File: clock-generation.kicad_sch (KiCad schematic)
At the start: 0 parts

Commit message: wip
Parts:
- added U1: Si5351B-B-GM, Package_DFN_QFN:QFN-20-1EP_4x4mm_P0.5mm_EP2.7x2.7mm, symbol Oscillator:Si5351B-B-GM
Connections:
- new net SCL: U1.4 (SCL)
- new net SDA: U1.5 (SDA)
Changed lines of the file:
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@@
 	(generator_version "8.0")
 	(paper "A4")
+	(wire
+		(pts
+			(xy 92.71 83.82) (xy 121.92 83.82)
+		)
+		(stroke
+			(width 0)
+			(type default)
+		)
+	)
+	(wire
+		(pts
+			(xy 92.71 86.36) (xy 121.92 86.36)
+		)
+		(stroke
+			(width 0)
+			(type default)
+		)
+	)
+	(hierarchical_label "SCL"
+		(shape bidirectional)
+		(at 92.71 86.36 180)
+		(fields_autoplaced yes)
+		(effects
+			(font
+				(size 1.27 1.27)
+			)
+			(justify right)
+		)
+	)
+	(hierarchical_label "SDA"
+		(shape bidirectional)
+		(at 92.71 83.82 180)
+		(fields_autoplaced yes)
+		(effects
+			(font
+				(size 1.27 1.27)
+			)
+			(justify right)
+		)
+	)
+	(symbol
+		(lib_id "Oscillator:Si5351B-B-GM")
+		(at 137.16 78.74 0)
+		(unit 1)
+		(exclude_from_sim no)
+		(in_bom yes)
+		(on_board yes)
+		(dnp no)
+		(fields_autoplaced yes)
+		(property "Reference" "U1"
+			(at 139.3541 101.6 0)
+			(effects
+				(font
+					(size 1.27 1.27)
+				)
+				(justify left)
+			)
+		)
+		(property "Value" "Si5351B-B-GM"
+			(at 139.3541 104.14 0)
+			(effects
+				(font
+					(size 1.27 1.27)
+				)
+				(justify left)
+			)
+		)
+		(property "Footprint" "Package_DFN_QFN:QFN-20-1EP_4x4mm_P0.5mm_EP2.7x2.7mm"
+			(at 137.16 109.22 0)
+			(effects
+				(font
+					(size 1.27 1.27)
+				)
+				(hide yes)
+			)
+		)
+		(property "Datasheet" "https://www.silabs.com/documents/public/data-sheets/Si5351-B.pdf"
+			(at 137.16 78.74 0)
+			(effects
+				(font
+					(size 1.27 1.27)
+				)
+				(hide yes)
+			)
+		)
+		(property "Description" "I2C Programmable Any-Frequency CMOS Clock Generator + VCXO, QFN-20"
+			(at 137.16 78.74 0)
+			(effects
+				(font
+					(size 1.27 1.27)
+				)
+				(hide yes)
+			)
+		)
+		(pin "17"
+		)
+		(pin "21"
+		)
+		(pin "20"
+		)
+		(pin "2"
+		)
+		(pin "3"
+		)
+		(pin "9"
+		)
+		(pin "1"
+		)
+		(pin "13"
+		)
+		(pin "5"
+		)
+		(pin "7"
+		)
+		(pin "4"
+		)
+		(pin "6"
+		)
+		(pin "15"
+		)
+		(pin "10"
+		)
+		(pin "8"
+		)
+		(pin "14"
+		)
+		(pin "18"
+		)
+		(pin "11"
+		)
+		(pin "16"
+		)
+		(pin "12"
+		)
+		(pin "19"
+		)
+		(instances
+			(project ""
+				(path "/df100556-b288-4cb1-b69f-c0734132cb90/be7c4f40-c0c2-47f2-9c0c-8904af6555df"
+					(reference "U1")
+					(unit 1)
+				)
+			)
+		)
+	)
 )

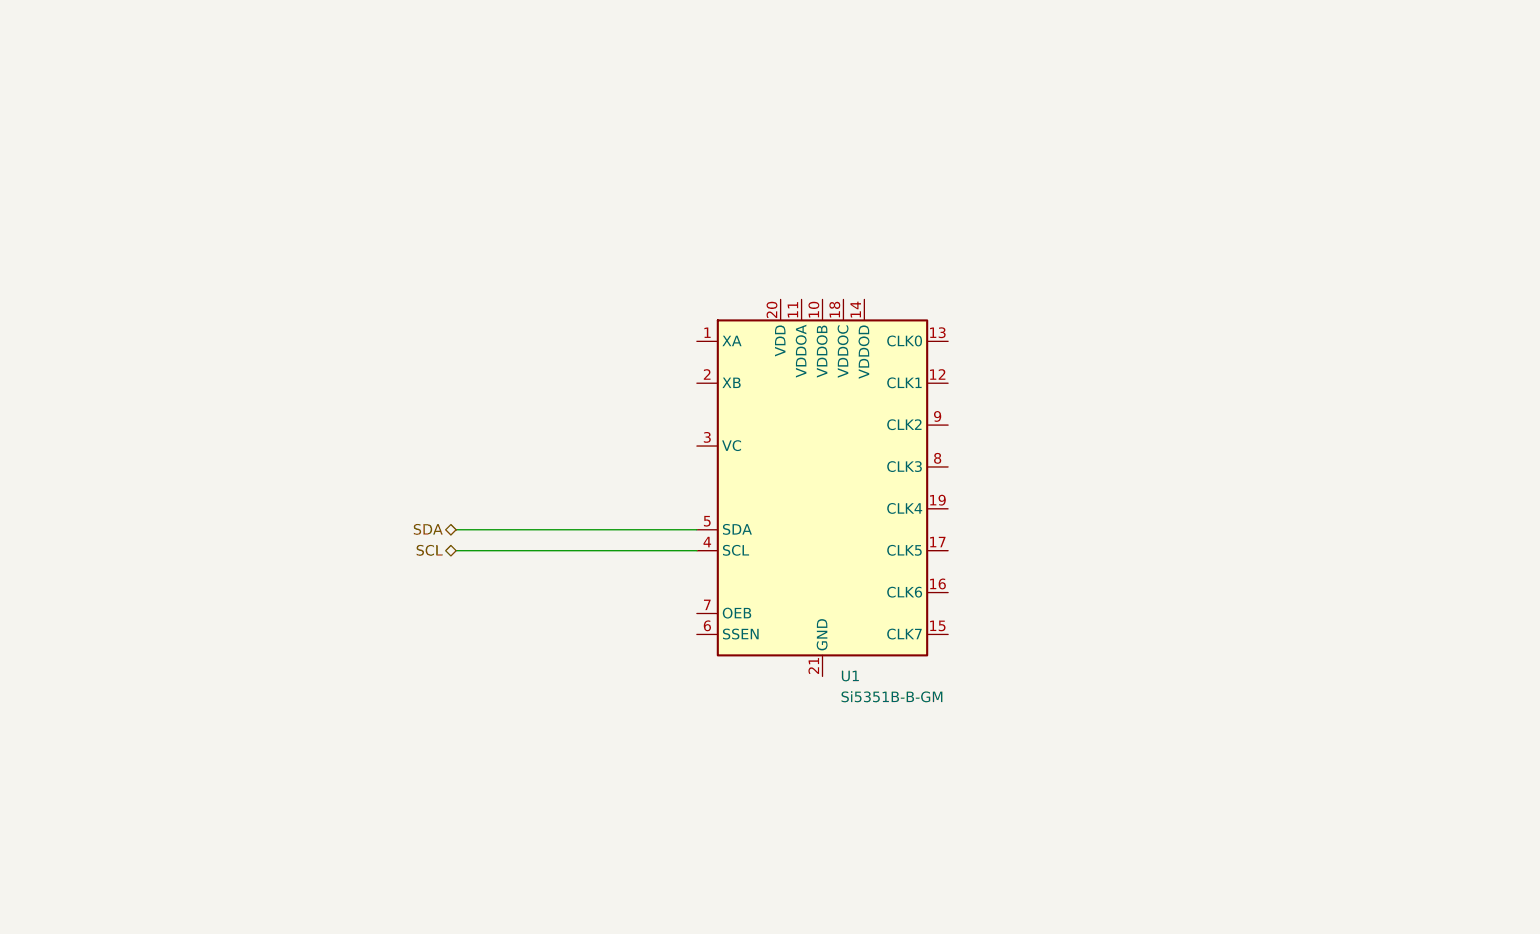
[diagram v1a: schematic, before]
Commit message: wip
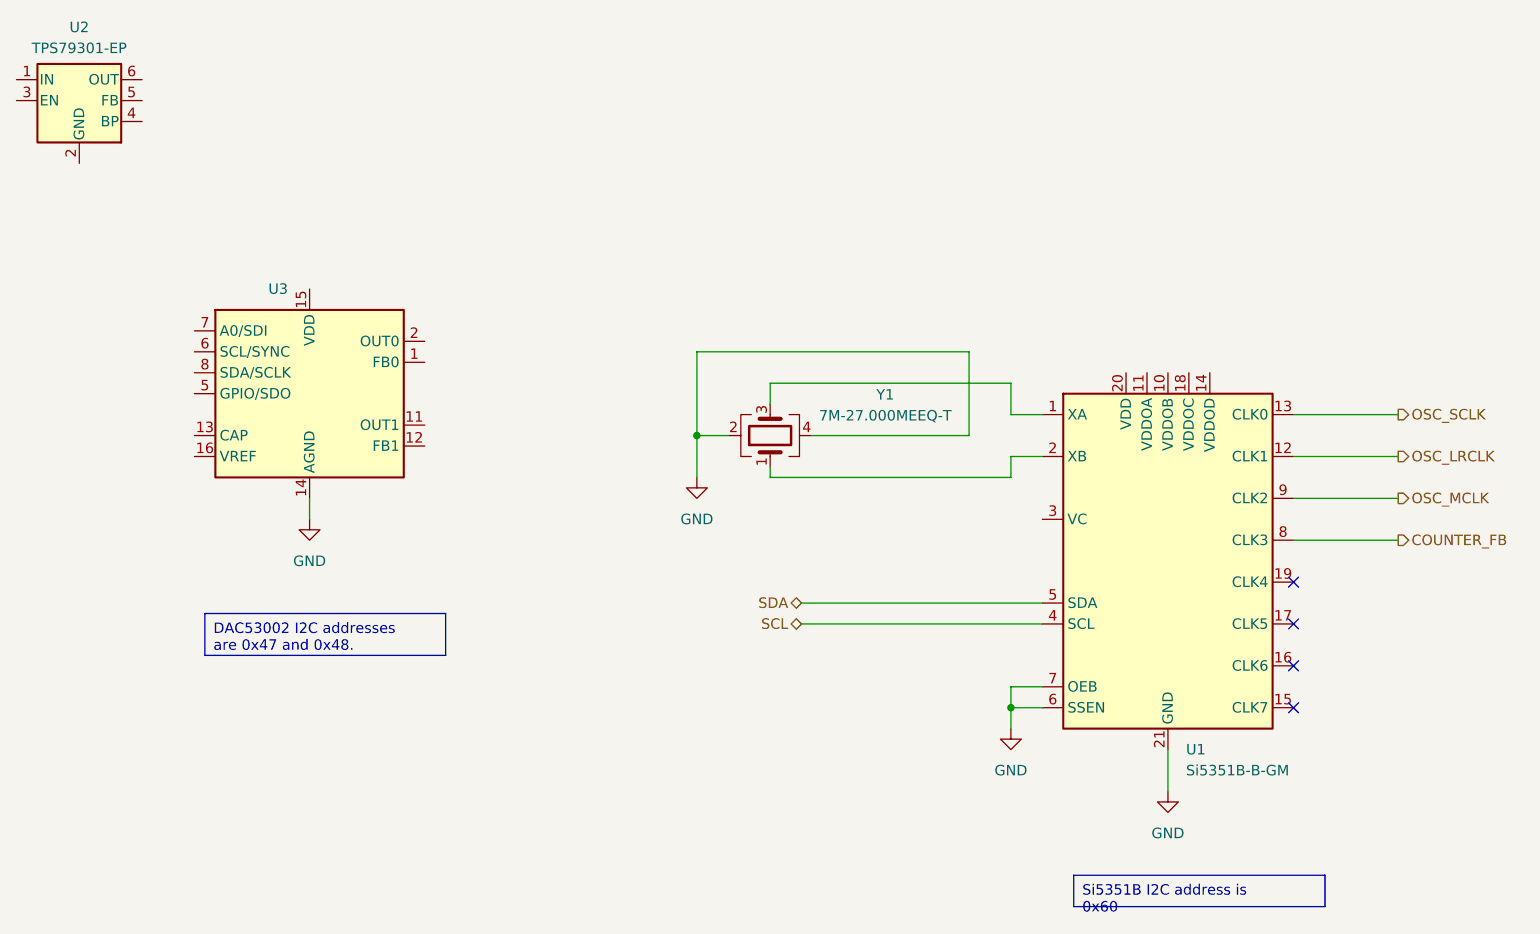
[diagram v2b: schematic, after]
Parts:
- added U2: TPS79301-EP, Package_TO_SOT_SMD:SOT-23-6, symbol Regulator_Linear:TPS79301-EP
- added U3: ~, symbol dante-audio-board:DAC53002
- added Y1: 7M-27.000MEEQ-T, Crystal:Crystal_SMD_TXC_7M-4Pin_3.2x2.5mm, symbol Device:Crystal_GND24
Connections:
- net at U1.1 (XA): now also Y1.3
- net OSC_LRCLK: now reaches U1.12 (CLK1)
- net OSC_SCLK: now reaches U1.13 (CLK0)
- net at U1.2 (XB): now also Y1.1
- net GND: now reaches U1.21 (GND)
- net GND: now also U1.6 (SSEN), U1.7 (OEB), U3.14 (AGND), Y1.2, Y1.4
- net COUNTER_FB: now reaches U1.8 (CLK3)
- net OSC_MCLK: now reaches U1.9 (CLK2)
- no-connect marks 0 -> 4
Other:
- moved on the sheet: U1
